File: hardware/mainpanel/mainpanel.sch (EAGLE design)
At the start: 16 parts, among them J1 CDH, J2 OW, J3 DBG, J4 SUN-UART, J5 ADCS, J6 ENV, J7 SUN, U1 DS18B20, U2 DS18B20, U3 DS18B20

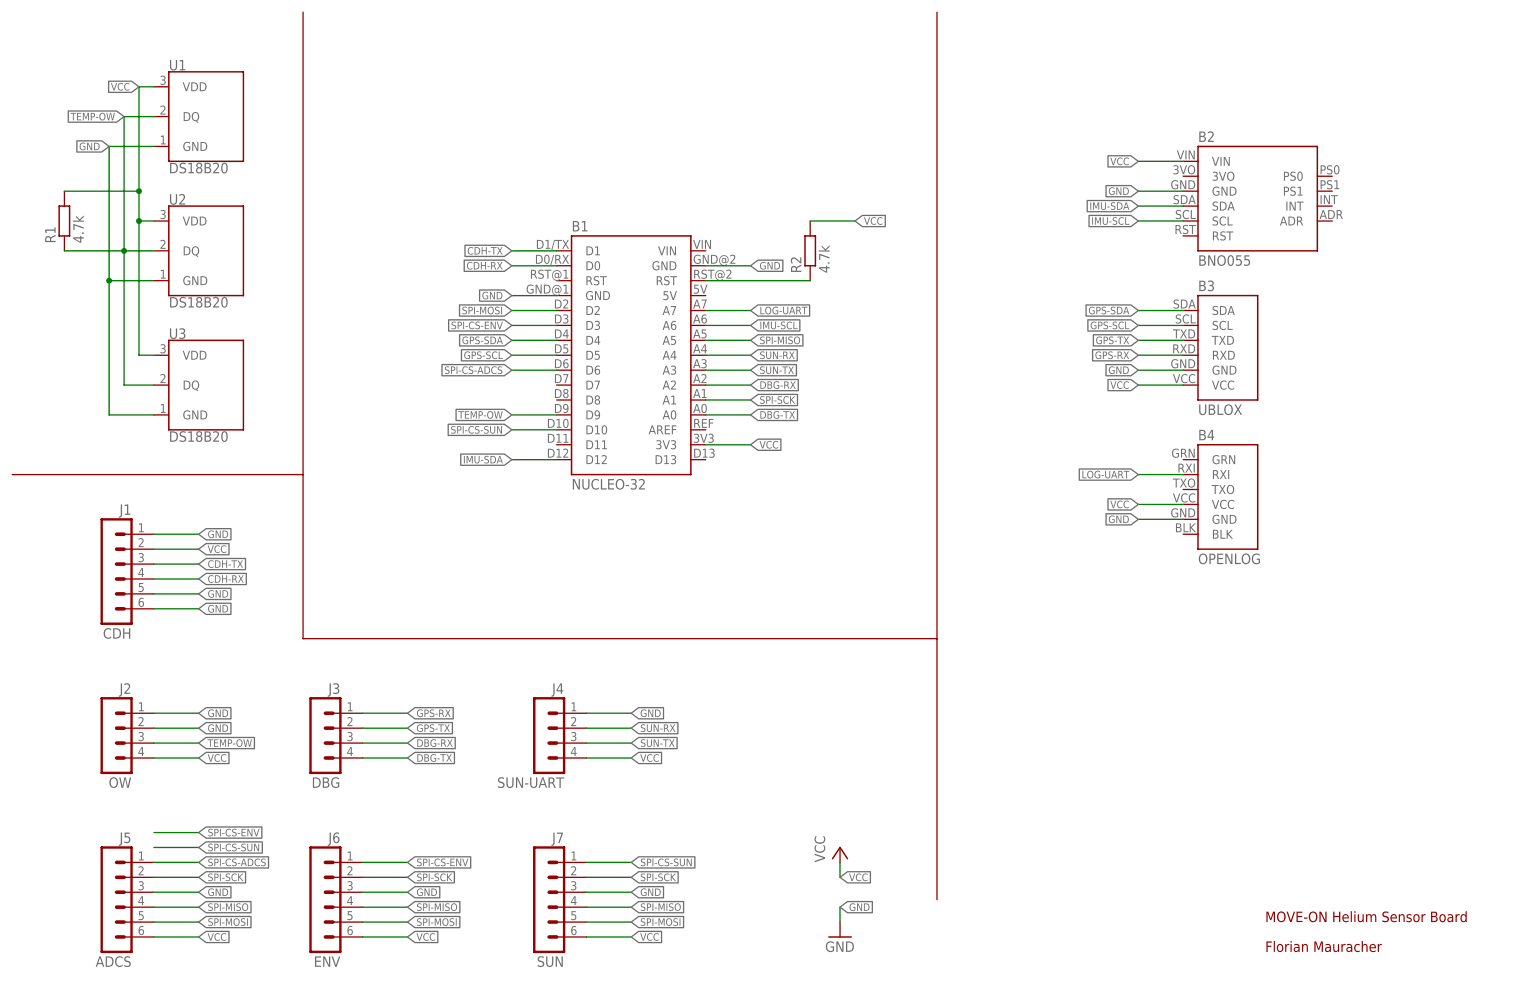
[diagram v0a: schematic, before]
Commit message: Move stuff
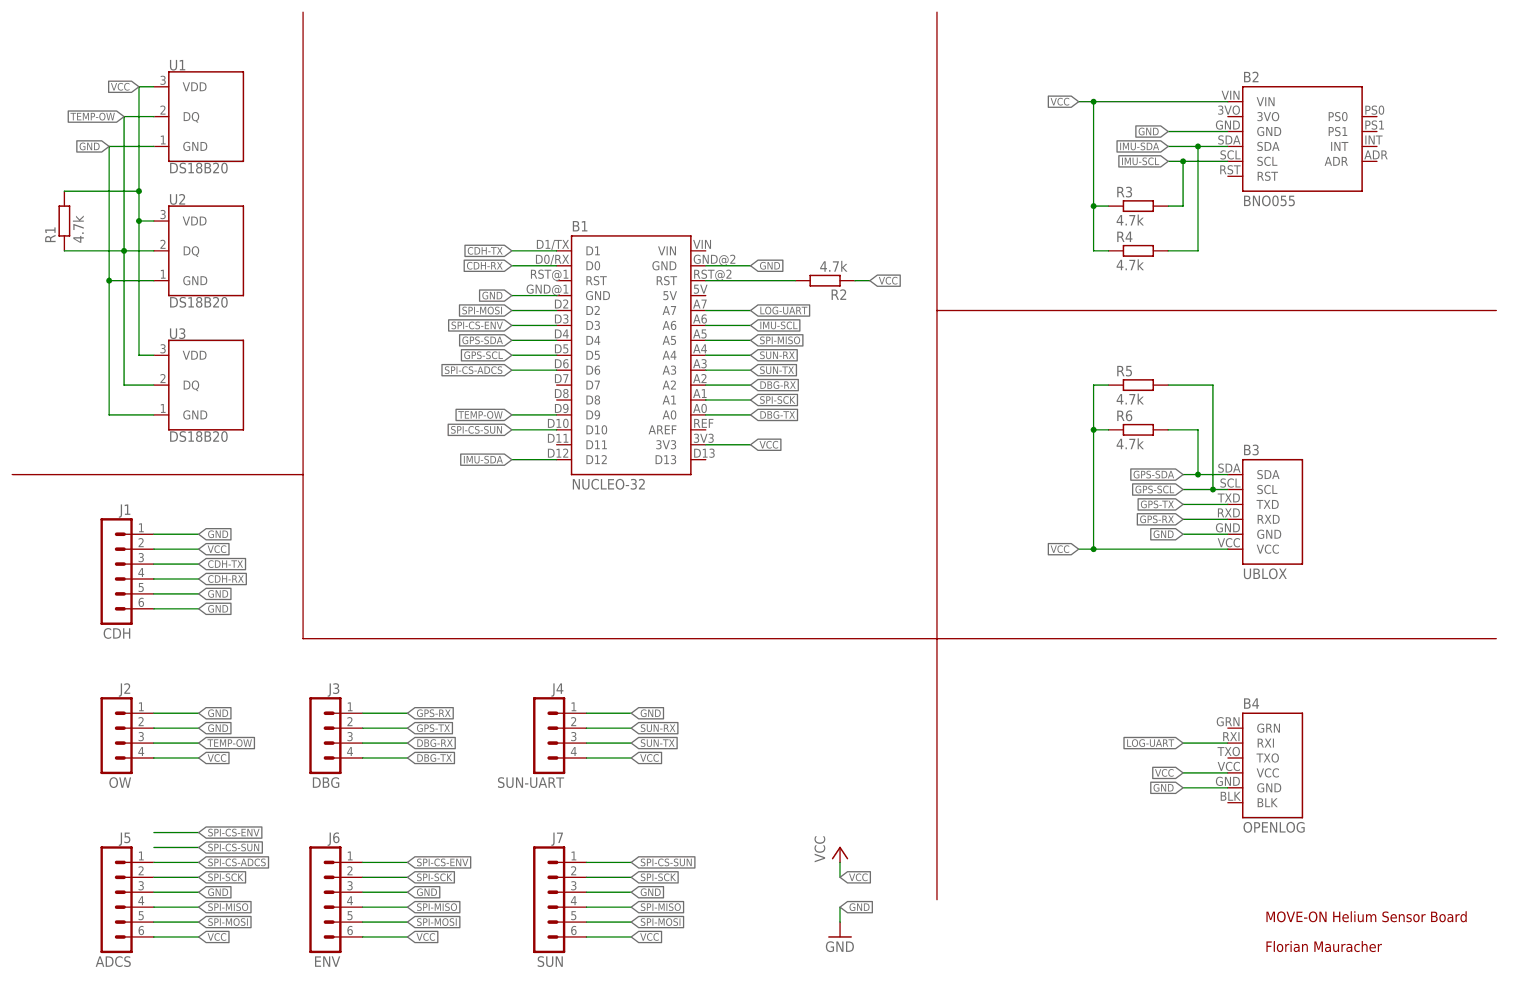
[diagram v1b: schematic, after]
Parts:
- added R3, R4, R5, R6: 4.7k, resistor:R-EU_M2012
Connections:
- net GPS-SCL: now also R5.2
- net GPS-SDA: now also R6.2
- net IMU-SCL: now also R3.2
- net IMU-SDA: now also R4.2
- net N$1: now also R2.2; no longer R2.1
- net VCC: now also R2.1, R3.1, R4.1, R5.1, R6.1; no longer R2.2
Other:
- moved on the sheet: B2, B3, B4, R2
